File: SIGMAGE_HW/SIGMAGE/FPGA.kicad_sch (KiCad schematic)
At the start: 52 parts, among them J9 TSW10607GS, U41 MMBT2222A, U8 LFE5U25F6BG256I

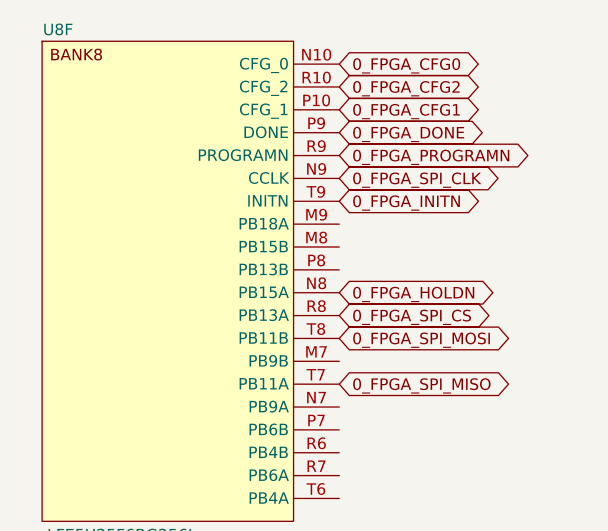
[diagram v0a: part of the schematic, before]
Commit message: some foo
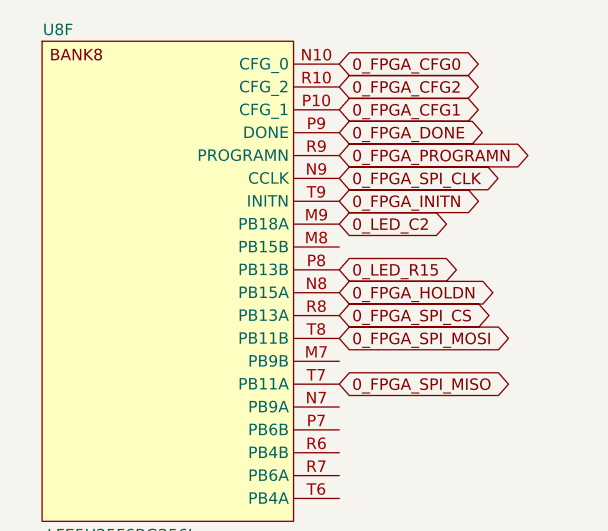
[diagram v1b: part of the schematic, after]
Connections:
- net 0_LED_C2: now also U8.M9 (PB18A)
- net 0_LED_R15: now also U8.P8 (PB13B)
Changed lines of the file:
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@@
 		)
 	)
+	(global_label "0_LED_R15"
+		(shape bidirectional)
+		(at 369.57 50.8 0)
+		(fields_autoplaced yes)
+		(effects
+			(font
+				(size 1.27 1.27)
+			)
+			(justify left)
+		)
+		(property "Intersheetrefs" "${INTERSHEET_REFS}"
+			(at 383.9473 50.8 0)
+			(hide yes)
+			(show_name no)
+			(do_not_autoplace no)
+			(effects
+				(font
+					(size 1.27 1.27)
+				)
+				(justify left)
+			)
+		)
+	)
 	(global_label "0_ICOM_AUX3"
 		(shape bidirectional)
@@
 			(hide yes)
 			(show_name no)
+			(do_not_autoplace no)
+			(effects
+				(font
+					(size 1.27 1.27)
+				)
+				(justify left)
+			)
+		)
+	)
+	(global_label "0_LED_C2"
+		(shape bidirectional)
+		(at 369.57 45.72 0)
+		(fields_autoplaced yes)
+		(effects
+			(font
+				(size 1.27 1.27)
+			)
+			(justify left)
+		)
+		(property "Intersheetrefs" "${INTERSHEET_REFS}"
+			(at 382.7378 45.72 0)
+			(hide yes)
+			(show_name no)

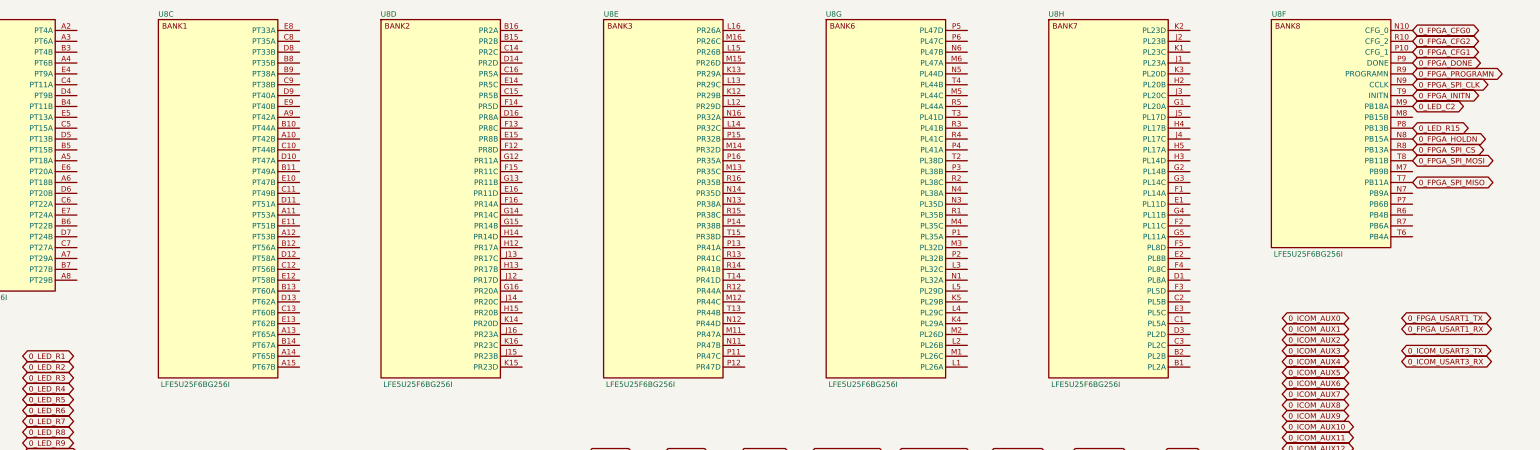
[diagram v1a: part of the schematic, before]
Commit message: more foo
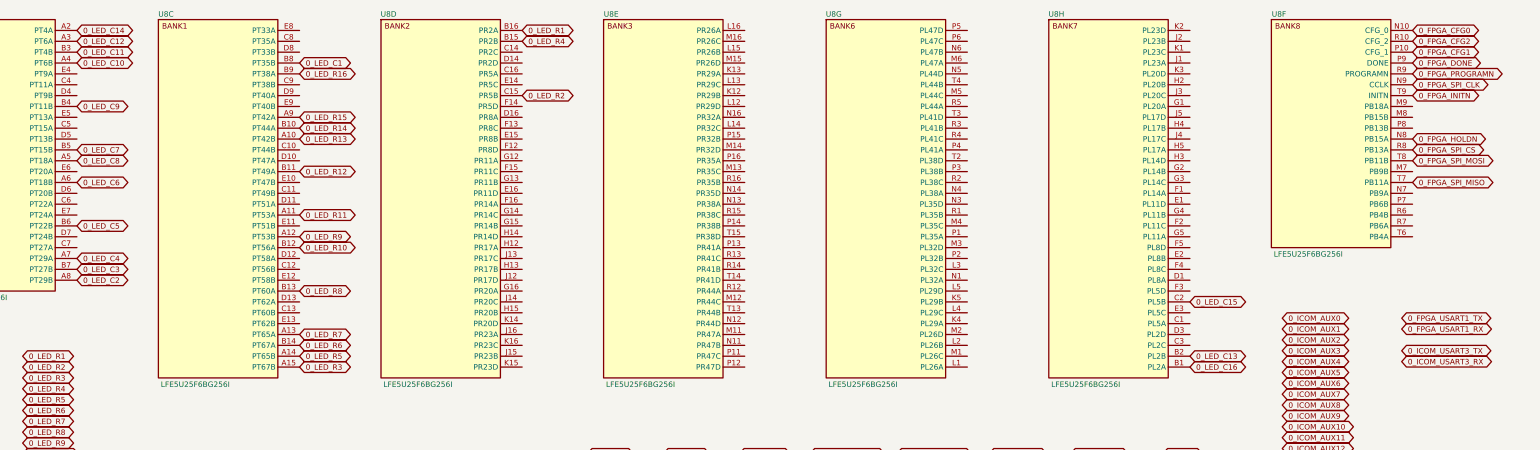
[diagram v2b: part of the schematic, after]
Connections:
- net 0_LED_C1: now also U8.B8 (PT35B)
- net 0_LED_C10: now also U8.A4 (PT6B)
- net 0_LED_C11: now also U8.B3 (PT4B)
- net 0_LED_C12: now also U8.A3 (PT6A)
- net 0_LED_C13: now also U8.B2 (PL2B)
- net 0_LED_C14: now also U8.A2 (PT4A)
- net 0_LED_C15: now also U8.C2 (PL5B)
- net 0_LED_C16: now also U8.B1 (PL2A)
- net 0_LED_C2: now also U8.A8 (PT29B); no longer U8.M9 (PB18A)
- net 0_LED_C3: now also U8.B7 (PT27B)
- net 0_LED_C4: now also U8.A7 (PT29A)
- net 0_LED_C5: now also U8.B6 (PT22B)
- net 0_LED_C6: now also U8.A6 (PT18B)
- net 0_LED_C7: now also U8.B5 (PT15B)
- net 0_LED_C8: now also U8.A5 (PT18A)
- net 0_LED_C9: now also U8.B4 (PT11B)
- net 0_LED_R1: now also U8.B16 (PR2A)
- net 0_LED_R10: now also U8.B12 (PT56A)
- net 0_LED_R11: now also U8.A11 (PT53A)
- net 0_LED_R12: now also U8.B11 (PT49A)
- net 0_LED_R13: now also U8.A10 (PT42B)
- net 0_LED_R14: now also U8.B10 (PT44A)
- net 0_LED_R15: now also U8.A9 (PT42A); no longer U8.P8 (PB13B)
- net 0_LED_R16: now also U8.B9 (PT38A)
- net 0_LED_R2: now also U8.C15 (PR5B)
- net 0_LED_R3: now also U8.A15 (PT67B)
- net 0_LED_R4: now also U8.B15 (PR2B)
- net 0_LED_R5: now also U8.A14 (PT65B)
- net 0_LED_R6: now also U8.B14 (PT67A)
- net 0_LED_R7: now also U8.A13 (PT65A)
- net 0_LED_R8: now also U8.B13 (PT60A)
- net 0_LED_R9: now also U8.A12 (PT53B)
